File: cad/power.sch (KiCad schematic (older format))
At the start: 29 parts, among them SW1 SW_PUSH, U3 TPS73001, U4 TPS73001

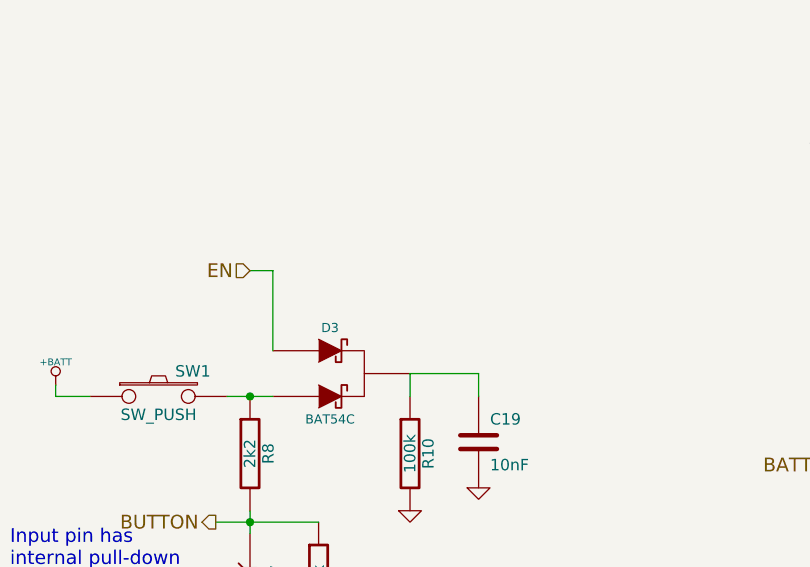
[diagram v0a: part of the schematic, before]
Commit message: whole bunch of stuff
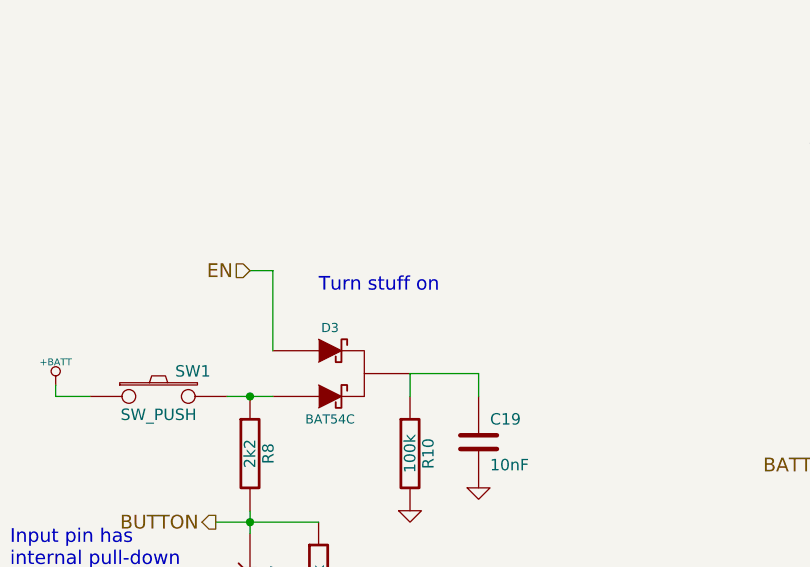
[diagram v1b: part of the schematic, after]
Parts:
- C17, C21, C26, C27: footprint (none) -> Capacitors_SMD:C_0603
- C18, C19, C20, C22, C23, C24, C25: footprint (none) -> Capacitors_SMD:C_0402
- SW1: MPN (none) -> PTS840 GM SMTR LFS
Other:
- note added: "Turn stuff on"
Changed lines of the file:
@@
 F 0 "C20" H 4000 2700 50  0000 L CNN
 F 1 "1uF" H 4000 2500 50  0000 L CNN
-F 2 "" H 3950 2600 60  0000 C CNN
+F 2 "Capacitors_SMD:C_0402" H 3950 2600 60  0001 C CNN
 F 3 "" H 3950 2600 60  0000 C CNN
 	1    3950 2600
@@
 F 0 "BT1" H 6850 6350 50  0000 C CNN
 F 1 "BATTERY" H 6850 5960 50  0000 C CNN
-F 2 "" H 6850 6150 60  0000 C CNN
+F 2 "" H 6850 6150 60  0001 C CNN
 F 3 "" H 6850 6150 60  0000 C CNN
 	1    6850 6150
@@
 F 0 "C22" H 4750 3400 50  0000 L CNN
 F 1 "10nF" H 4750 3200 50  0000 L CNN
-F 2 "" H 4700 3300 60  0000 C CNN
+F 2 "Capacitors_SMD:C_0402" H 4700 3300 60  0001 C CNN
 F 3 "" H 4700 3300 60  0000 C CNN
 	1    4700 3300
@@
 F 0 "C26" H 7050 2700 50  0000 L CNN
 F 1 "4.7uF" H 7050 2500 50  0000 L CNN
-F 2 "" H 7000 2600 60  0000 C CNN
+F 2 "Capacitors_SMD:C_0603" H 7000 2600 60  0001 C CNN
 F 3 "" H 7000 2600 60  0000 C CNN
 F 4 "CL10B475KQ8NQNC" H 7000 2600 60  0001 C CNN "MPN"
@@
 F 0 "R14" V 5630 3200 50  0000 C CNN
 F 1 "0" V 5550 3200 50  0000 C CNN
-F 2 "" H 5550 3200 60  0000 C CNN
+F 2 "" H 5550 3200 60  0001 C CNN
 F 3 "" H 5550 3200 60  0000 C CNN
 F 4 "RC1005J000CS" V 5550 3200 60  0001 C CNN "MPN"
@@
 F 0 "R16" V 6280 2650 50  0000 C CNN
 F 1 "39k" V 6200 2650 50  0000 C CNN
-F 2 "" H 6200 2650 60  0000 C CNN
+F 2 "" H 6200 2650 60  0001 C CNN
 F 3 "" H 6200 2650 60  0000 C CNN
 F 4 "RC1005J393CS" V 6200 2650 60  0001 C CNN "MPN"
@@
 F 0 "R17" V 6280 3250 50  0000 C CNN
 F 1 "30k" V 6200 3250 50  0000 C CNN
-F 2 "" H 6200 3250 60  0000 C CNN
+F 2 "" H 6200 3250 60  0001 C CNN
 F 3 "" H 6200 3250 60  0000 C CNN
 F 4 "RC1005J303CS" V 6200 3250 60  0001 C CNN "MPN"
@@
 F 0 "C24" H 6550 2750 50  0000 L CNN
 F 1 "22pF" H 6550 2550 50  0000 L CNN
-F 2 "" H 6500 2650 60  0000 C CNN
+F 2 "Capacitors_SMD:C_0402" H 6500 2650 60  0001 C CNN
 F 3 "" H 6500 2650 60  0000 C CNN
 F 4 "CL05C220JB5NNNC" H 6500 2650 60  0001 C CNN "MPN"
@@
 F 0 "C21" H 4000 4250 50  0000 L CNN
 F 1 "4.7uF" H 4000 4050 50  0000 L CNN
-F 2 "" H 3950 4150 60  0000 C CNN
+F 2 "Capacitors_SMD:C_0603" H 3950 4150 60  0001 C CNN
 F 3 "" H 3950 4150 60  0000 C CNN
 	1    3950 4150
@@
 F 0 "C23" H 4750 4950 50  0000 L CNN
 F 1 "10nF" H 4750 4750 50  0000 L CNN
-F 2 "" H 4700 4850 60  0000 C CNN
+F 2 "Capacitors_SMD:C_0402" H 4700 4850 60  0001 C CNN
 F 3 "" H 4700 4850 60  0000 C CNN
 	1    4700 4850
@@
 F 0 "C27" H 7050 4250 50  0000 L CNN
 F 1 "4.7uF" H 7050 4050 50  0000 L CNN
-F 2 "" H 7000 4150 60  0000 C CNN
+F 2 "Capacitors_SMD:C_0603" H 7000 4150 60  0001 C CNN
 F 3 "" H 7000 4150 60  0000 C CNN
 	1    7000 4150
@@
 F 0 "R15" V 5630 4750 50  0000 C CNN
 F 1 "0" V 5550 4750 50  0000 C CNN
-F 2 "" H 5550 4750 60  0000 C CNN
+F 2 "" H 5550 4750 60  0001 C CNN
 F 3 "" H 5550 4750 60  0000 C CNN
 	1    5550 4750
@@
 F 0 "R18" V 6280 4200 50  0000 C CNN
 F 1 "39k" V 6200 4200 50  0000 C CNN
-F 2 "" H 6200 4200 60  0000 C CNN
+F 2 "" H 6200 4200 60  0001 C CNN
 F 3 "" H 6200 4200 60  0000 C CNN
 	1    6200 4200
@@
 F 0 "R19" V 6280 4800 50  0000 C CNN
 F 1 "30k" V 6200 4800 50  0000 C CNN
-F 2 "" H 6200 4800 60  0000 C CNN
+F 2 "" H 6200 4800 60  0001 C CNN
 F 3 "" H 6200 4800 60  0000 C CNN
 	1    6200 4800
@@
 F 0 "C25" H 6550 4300 50  0000 L CNN
 F 1 "22pF" H 6550 4100 50  0000 L CNN
-F 2 "" H 6500 4200 60  0000 C CNN
+F 2 "Capacitors_SMD:C_0402" H 6500 4200 60  0001 C CNN
 F 3 "" H 6500 4200 60  0000 C CNN
 	1    6500 4200
@@
 F 0 "R11" V 3630 3950 50  0000 C CNN
 F 1 "10" V 3550 3950 50  0000 C CNN
-F 2 "" H 3550 3950 60  0000 C CNN
+F 2 "" H 3550 3950 60  0001 C CNN
 F 3 "" H 3550 3950 60  0000 C CNN
 F 4 "MCR01MRTF10R0" V 3550 3950 60  0001 C CNN "MPN"
@@
 F 0 "C17" H 2850 4250 50  0000 L CNN
 F 1 "4.7uF" H 2850 4050 50  0000 L CNN
-F 2 "" H 2800 4150 60  0000 C CNN
+F 2 "Capacitors_SMD:C_0603" H 2800 4150 60  0001 C CNN
 F 3 "" H 2800 4150 60  0000 C CNN
 	1    2800 4150
@@
 F 0 "C18" H 3200 4250 50  0000 L CNN
 F 1 "100nF" H 3200 4050 50  0000 L CNN
-F 2 "" H 3150 4150 60  0000 C CNN
+F 2 "Capacitors_SMD:C_0402" H 3150 4150 60  0001 C CNN
 F 3 "" H 3150 4150 60  0000 C CNN
 	1    3150 4150
@@
 F 0 "SW1" H 1900 6360 50  0000 C CNN
 F 1 "SW_PUSH" H 1750 6170 50  0000 C CNN
-F 2 "" H 1750 6250 60  0000 C CNN
+F 2 "" H 1750 6250 60  0001 C CNN
 F 3 "" H 1750 6250 60  0000 C CNN
+F 4 "PTS840 GM SMTR LFS" H 1750 6250 60  0001 C CNN "MPN"
 	1    1750 6250
 	1    0    0    -1
@@
 F 0 "R10" V 2930 6500 50  0000 C CNN
 F 1 "100k" V 2850 6500 50  0000 C CNN
-F 2 "" H 2850 6500 60  0000 C CNN
+F 2 "" H 2850 6500 60  0001 C CNN
 F 3 "" H 2850 6500 60  0000 C CNN
 F 4 "MCR01MRTF1003" V 2850 6500 60  0001 C CNN "MPN"
@@
 F 0 "D2" H 2150 7150 50  0000 C CNN
 F 1 "2.7v" H 2150 6950 40  0000 C CNN
-F 2 "" H 2150 7050 60  0000 C CNN
+F 2 "" H 2150 7050 60  0001 C CNN
 F 3 "" H 2150 7050 60  0000 C CNN
 F 4 "MM3Z2V7T1G" H 2150 7050 60  0001 C CNN "MPN"
@@
 F 0 "R8" V 2230 6500 50  0000 C CNN
 F 1 "2k2" V 2150 6500 50  0000 C CNN
-F 2 "" H 2150 6500 60  0000 C CNN
+F 2 "" H 2150 6500 60  0001 C CNN
 F 3 "" H 2150 6500 60  0000 C CNN
 F 4 "RMCF0402JT2K20" V 2150 6500 60  0001 C CNN "MPN"
@@
 F 0 "C19" H 3200 6550 50  0000 L CNN
 F 1 "10nF" H 3200 6350 50  0000 L CNN
-F 2 "" H 3150 6450 60  0000 C CNN
+F 2 "Capacitors_SMD:C_0402" H 3150 6450 60  0001 C CNN
 F 3 "" H 3150 6450 60  0000 C CNN
 	1    3150 6450
@@
 F 0 "R9" V 2530 7050 50  0000 C CNN
 F 1 "20k" V 2450 7050 50  0000 C CNN
-F 2 "" H 2450 7050 60  0000 C CNN
+F 2 "" H 2450 7050 60  0001 C CNN
 F 3 "" H 2450 7050 60  0000 C CNN
 F 4 "MCR01MRTF2002" V 2450 7050 60  0001 C CNN "MPN"
@@
 F 0 "R13" V 5380 6850 50  0000 C CNN
 F 1 "62k" V 5300 6850 50  0000 C CNN
-F 2 "" H 5300 6850 60  0000 C CNN
+F 2 "" H 5300 6850 60  0001 C CNN
 F 3 "" H 5300 6850 60  0000 C CNN
 F 4 "MCR01MRTJ623" V 5300 6850 60  0001 C CNN "MPN"
@@
 F 0 "R12" V 5380 6250 50  0000 C CNN
 F 1 "36k" V 5300 6250 50  0000 C CNN
-F 2 "" H 5300 6250 60  0000 C CNN
+F 2 "" H 5300 6250 60  0001 C CNN
 F 3 "" H 5300 6250 60  0000 C CNN
 F 4 "MCR01MRTF3602" V 5300 6250 60  0001 C CNN "MPN"
@@
 F 0 "D3" H 2500 6350 40  0000 C CNN
 F 1 "BAT54C" H 2500 5950 40  0000 C CNN
-F 2 "" H 2500 6300 60  0000 C CNN
+F 2 "" H 2500 6300 60  0001 C CNN
 F 3 "" H 2500 6300 60  0000 C CNN
 	1    2500 6150
@@
 F 0 "U3" H 5200 2750 60  0000 C CNN
 F 1 "TPS73001" H 5500 2250 60  0000 C CNN
-F 2 "" H 5250 2500 60  0000 C CNN
+F 2 "" H 5250 2500 60  0001 C CNN
 F 3 "" H 5250 2500 60  0000 C CNN
 F 4 "TPS73001DBVR" H 5250 2500 60  0001 C CNN "MPN"
@@
 F 0 "U4" H 5200 4300 60  0000 C CNN
 F 1 "TPS73001" H 5500 3800 60  0000 C CNN
-F 2 "" H 5250 4050 60  0000 C CNN
+F 2 "" H 5250 4050 60  0001 C CNN
 F 3 "" H 5250 4050 60  0000 C CNN
 	1    5250 4050
 	1    0    0    -1
 $EndComp
+Text Notes 2450 5800 0    60   ~ 0
+Turn stuff on
 $EndSCHEMATC

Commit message: more stuff
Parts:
- D3: footprint (none) -> Diodes_SMD:Diode_SOT23
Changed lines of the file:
@@
 F 0 "D3" H 2500 6350 40  0000 C CNN
 F 1 "BAT54C" H 2500 5950 40  0000 C CNN
-F 2 "" H 2500 6300 60  0001 C CNN
+F 2 "Diodes_SMD:Diode_SOT23" H 2500 6300 60  0001 C CNN
 F 3 "" H 2500 6300 60  0000 C CNN
 	1    2500 6150
